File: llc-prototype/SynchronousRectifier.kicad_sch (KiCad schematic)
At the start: 3 parts, among them U2 UCC24624DR

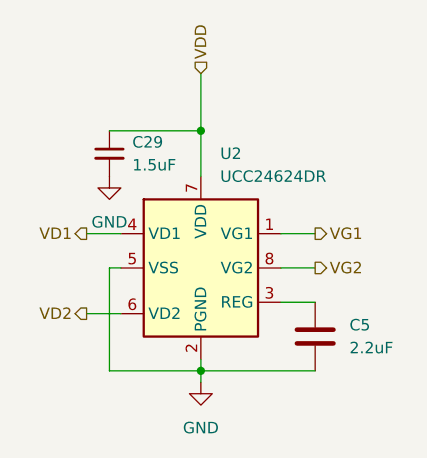
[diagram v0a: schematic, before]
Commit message: schematic
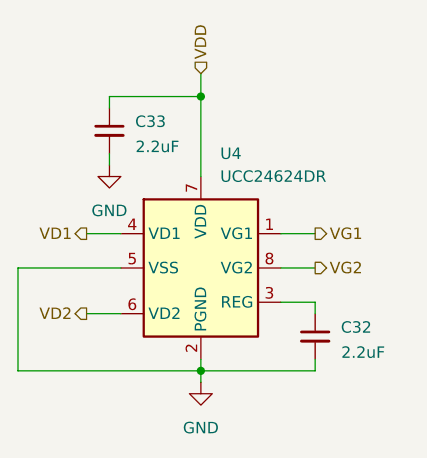
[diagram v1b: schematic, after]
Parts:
- removed C29: 1.5uF, Capacitor_SMD:C_0603_1608Metric_Pad1.08x0.95mm_HandSolder, symbol Device:C_Small
- removed C5: 2.2uF, Capacitor_SMD:C_0603_1608Metric_Pad1.08x0.95mm_HandSolder, symbol Device:C
- added C32, C33: 2.2uF, Capacitor_SMD:C_0603_1608Metric_Pad1.08x0.95mm_HandSolder, symbol Device:C_Small
- U4: renamed from U2; Digi PN 296-UCC24624DRCT-ND -> (none); Digi URL https://www.digikey.com/en/products/detail/texas-instrument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 -> (none); Digikey PN 296-UCC24624DRCT-ND -> (none); Digikey Part Number (none) -> 296-UCC24624DRCT-ND; MFG Texas Instruments -> (none); MFG PN UCC24624DR -> (none); Manufacturer (none) -> Texas Instruments; Manufacturer Part Number (none) -> UCC24624DR
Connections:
- net GND: now also C32.2, C33.2
- net VDD: now also C33.1
- net at U4.3 (REG): now also C32.1
